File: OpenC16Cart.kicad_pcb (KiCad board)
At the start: 2 copper layers, 57 x 62.5 mm, 14 parts, among them CN1 C16_EXP_PORT_44PIN, J1 Conn_02x03_Odd_Even, J2 Conn_02x03_Odd_Even, SW1 BTN_RESET, U1 27512

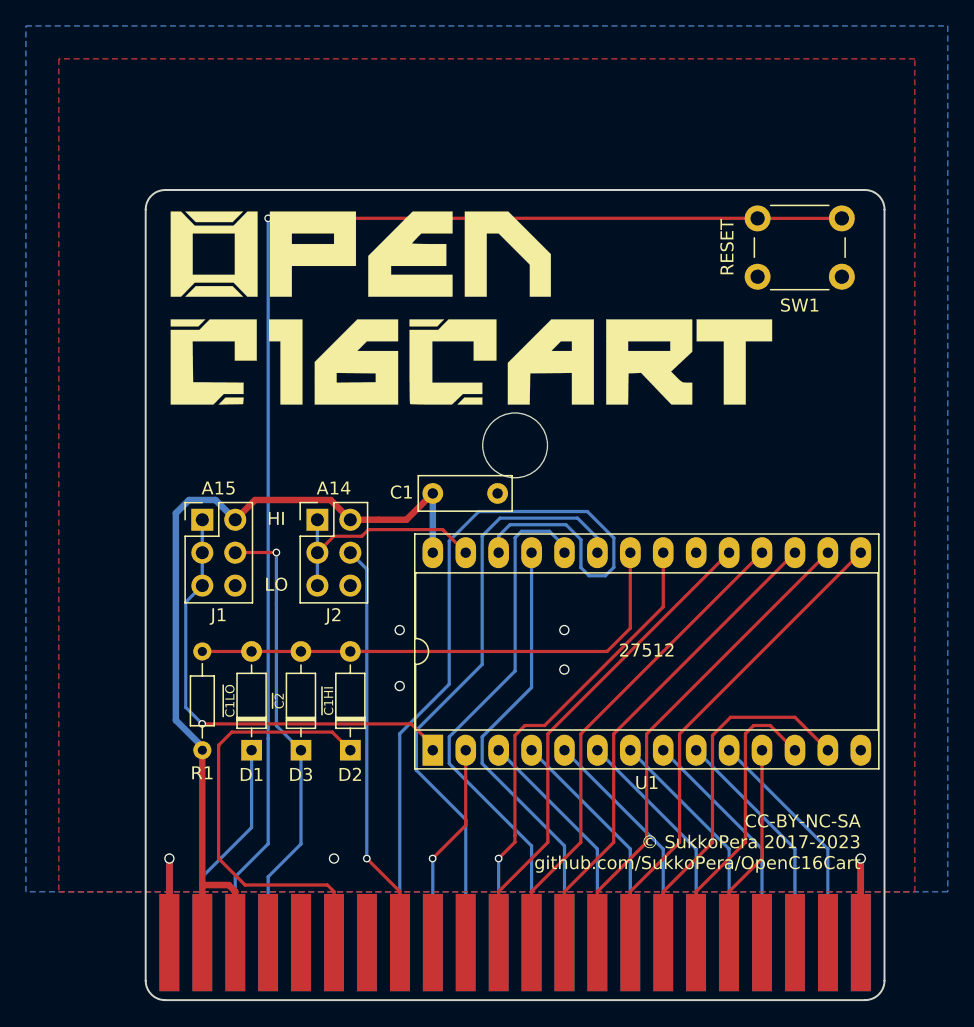
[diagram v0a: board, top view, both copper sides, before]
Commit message: Move components bottom left
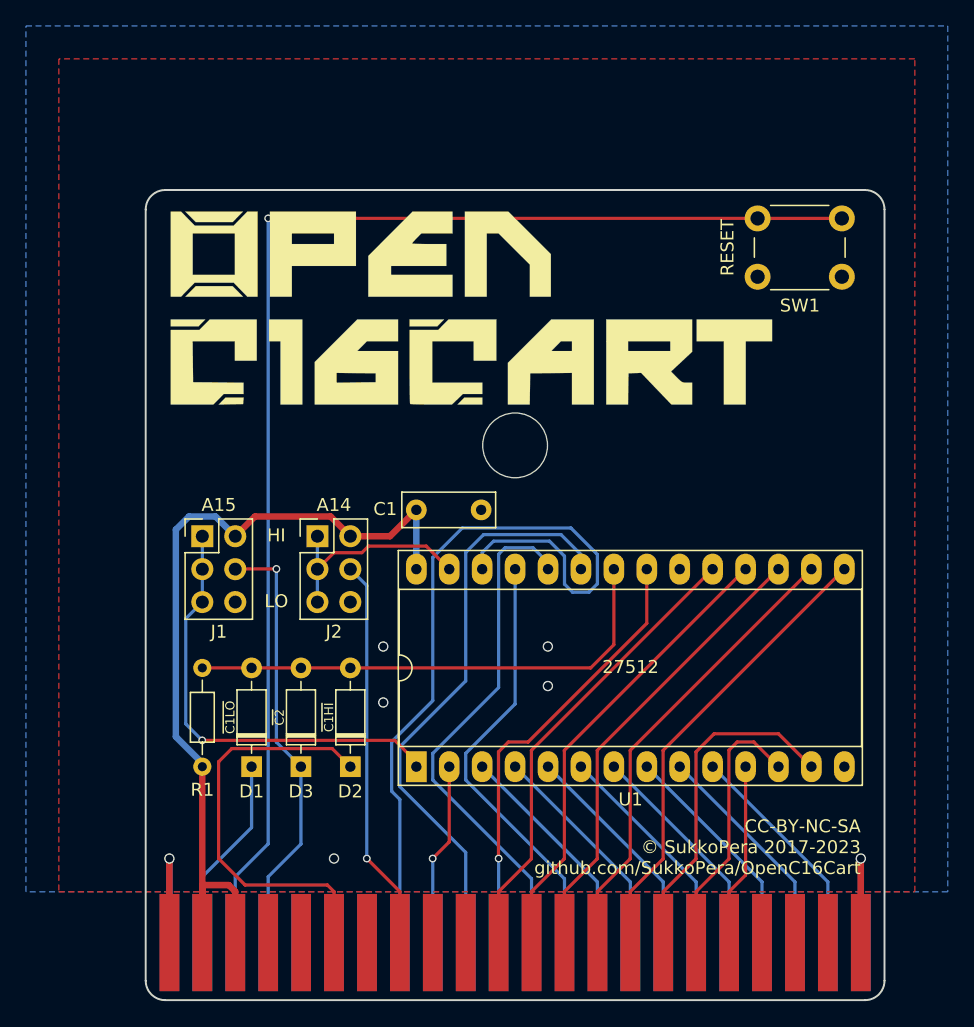
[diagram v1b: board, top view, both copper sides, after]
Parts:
- moved V0 1.80 mm to (158.4, 102.9)
- moved C1 1.80 mm to (141.9, 90.7)
- moved U1 1.80 mm to (141.9, 110.5)
- moved R1 1.27 mm to (125.4, 102.9)
- moved D1 1.27 mm to (129.2, 110.5)
- moved D2 1.27 mm to (136.8, 110.5)
- moved D3 1.27 mm to (133.0, 110.5)
- moved J1 1.27 mm to (125.4, 92.7)
- moved J2 1.27 mm to (134.2, 92.7)
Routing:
- net /a13: track 59.8 -> 62.1 mm
- net VCC: track 69.0 -> 70.9 mm
- net /d1: track 22.6 -> 20.8 mm
- net /d0: track 15.9 -> 14.1 mm
- net /a12: track 15.9 -> 14.1 mm
- net /d6: track 37.4 -> 35.6 mm
- net /d5: track 37.4 -> 35.6 mm
- net /d2: track 28.1 -> 26.3 mm
- net /d7: track 37.4 -> 35.6 mm
- net /d4: track 37.4 -> 35.6 mm
- net /d3: track 37.4 -> 35.6 mm
- net /a10: track 36.2 -> 34.4 mm
- net /~c1hi: track 33.8 -> 32.5 mm
- net /rom_a15: track 35.7 -> 34.4 mm
- net /~cs0: track 31.7 -> 30.4 mm
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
